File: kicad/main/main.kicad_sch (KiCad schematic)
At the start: 16 parts, among them J1 Conn_01x02, J3 Conn_01x07_Pin, J4 Conn_01x04_Pin, P1 USB_C_Plug_USB2.0, SW1 K3-1391B-51, SW3 SW_Push, SW4 SW_Push, U1 HUSB237

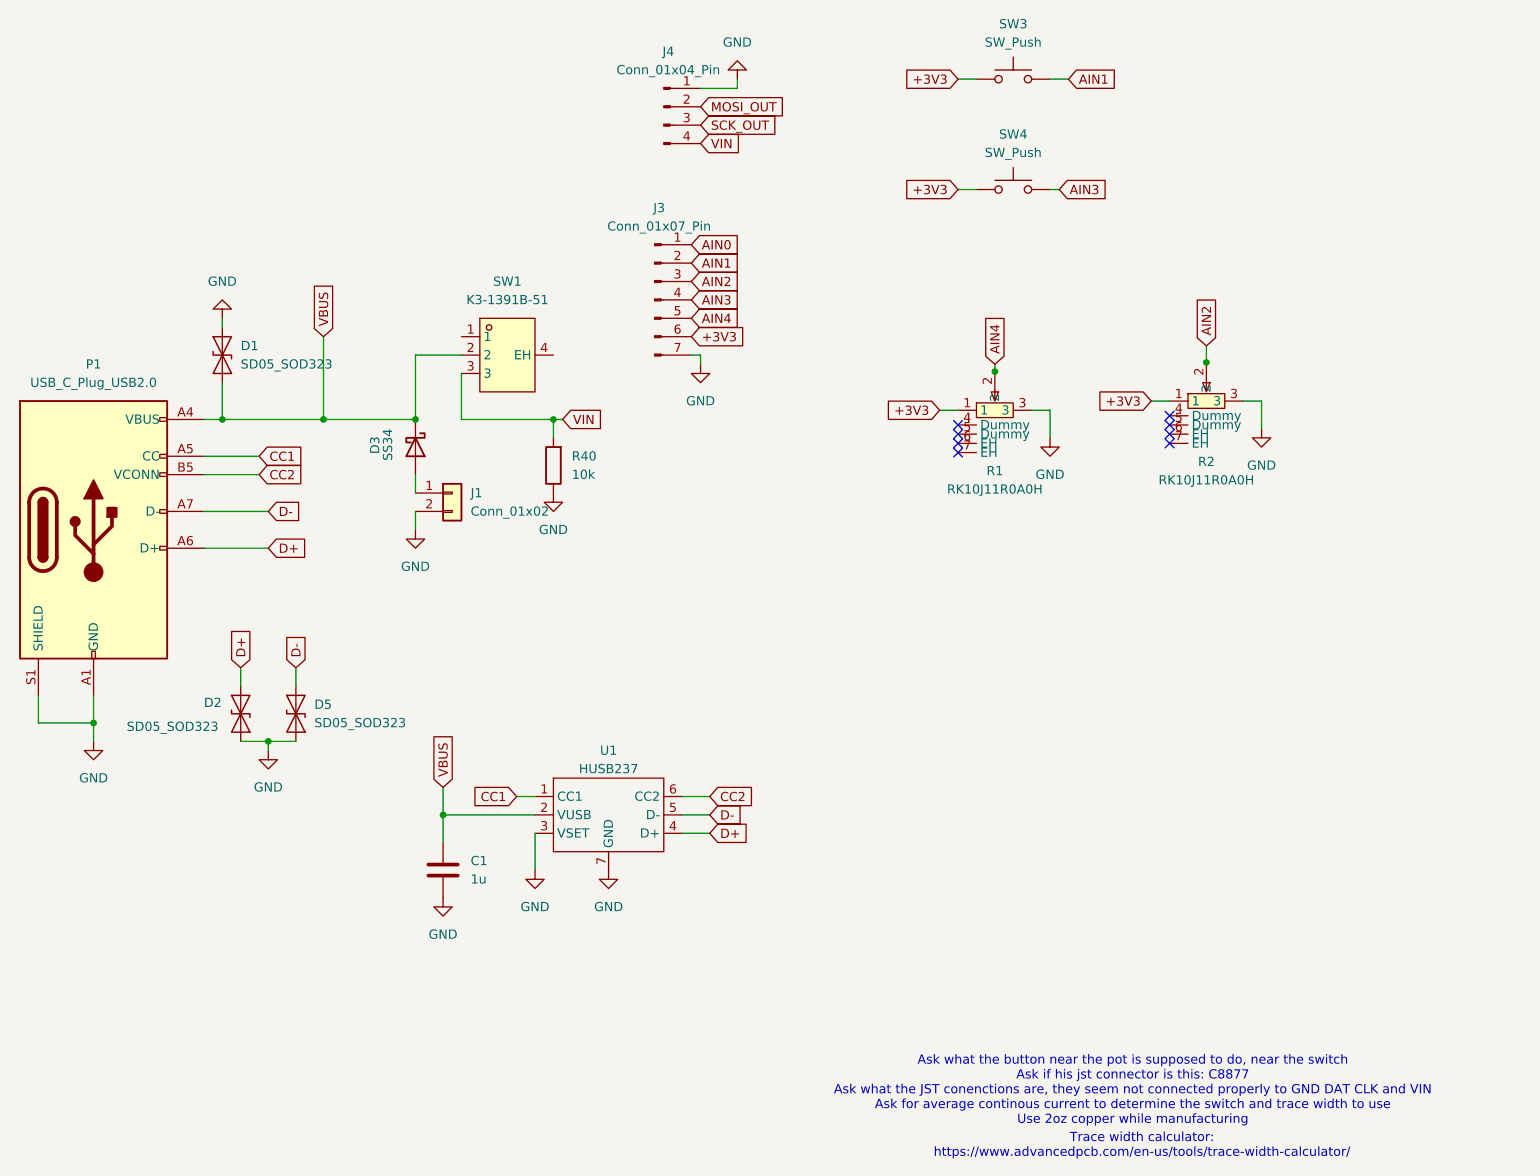
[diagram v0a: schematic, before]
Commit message: Finished design
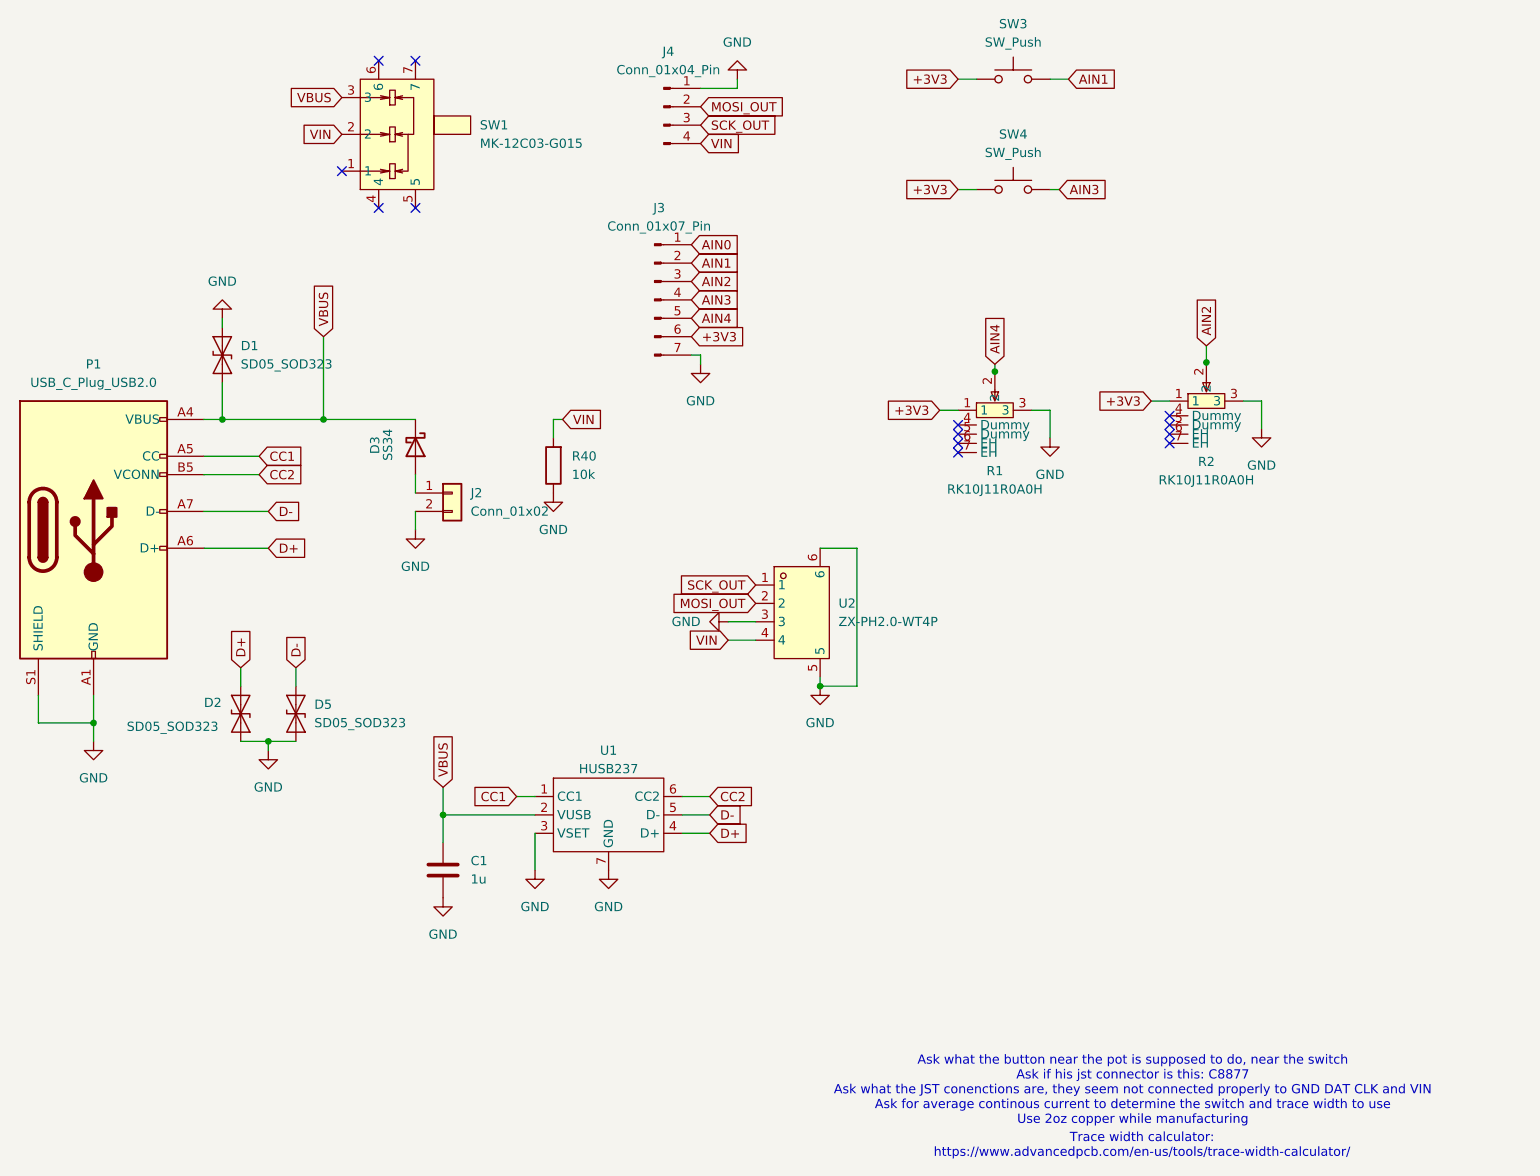
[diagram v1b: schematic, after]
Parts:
- removed SW1: K3-1391B-51, easyeda2kicad:SW-TH_K3-1391B-51, symbol easyeda2kicad:K3-1391B-51
- added SW1: MK-12C03-G015, easyeda2kicad:SW-SMD_MK-12C03-G015, symbol easyeda2kicad:MK-12C03-G015
- added U2: ZX-PH2.0-WT4P, easyeda2kicad:CONN-SMD_4P-P2.00_C2001RS10411M0101RC, symbol easyeda2kicad:ZX-PH2.0-WT4P
- C1: footprint (none) -> Capacitor_SMD:C_0805_2012Metric
- J2: renamed from J1; footprint (none) -> Connector_PinHeader_2.54mm:PinHeader_1x02_P2.54mm_Vertical
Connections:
- net GND: now also U2.3, U2.5, U2.6
- net MOSI_OUT: now also U2.2
- net SCK_OUT: now also U2.1
- net VBUS: now also SW1.3
- net VIN: now also SW1.2, U2.4
- no-connect marks 8 -> 13

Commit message: Rewired PCB
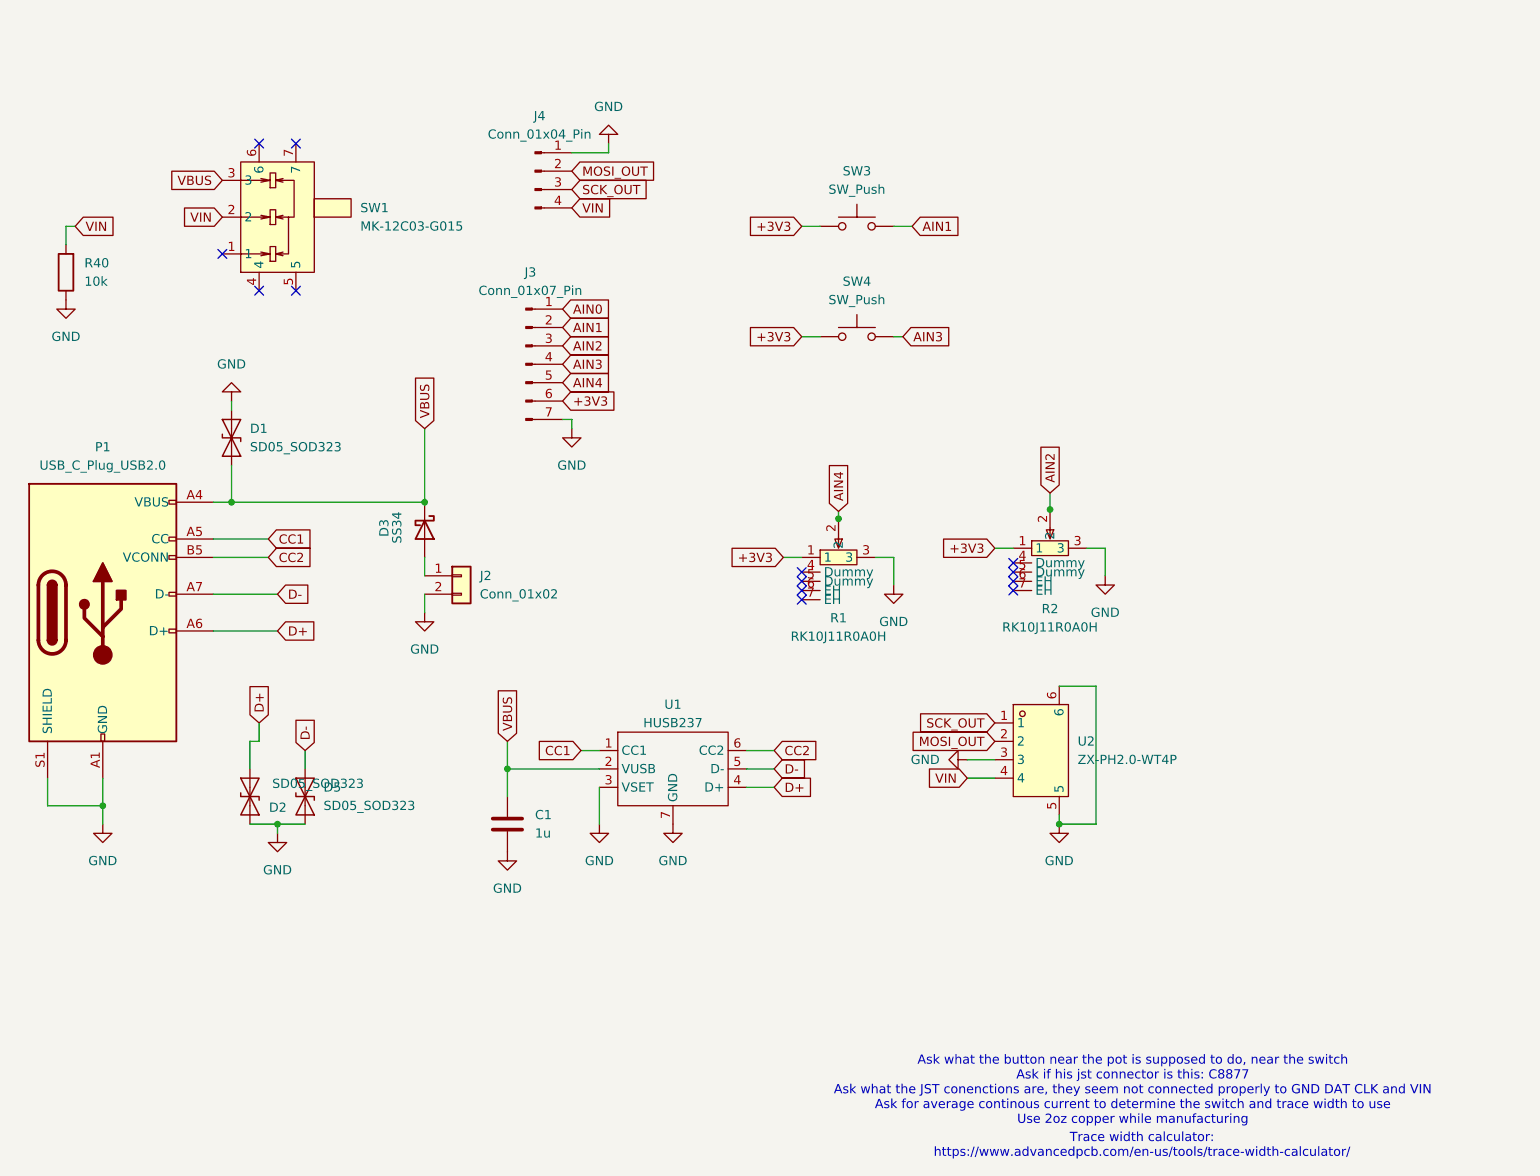
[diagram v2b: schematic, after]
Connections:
- net D+: now also D2.1 (A1); no longer D2.2 (A2)
- net D-: now also D5.1 (A1); no longer D5.2 (A2)
- net GND: now also D2.2 (A2), D5.2 (A2); no longer D2.1 (A1), D5.1 (A1)
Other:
- moved on the sheet: C1, D1, D2, D3, D5, J2, J3, J4, P1, R1, R2, R40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
